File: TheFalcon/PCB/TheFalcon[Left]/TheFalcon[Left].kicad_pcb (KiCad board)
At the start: 4 copper layers, 173.3 x 142.5 mm, 171 parts, among them IC1 IS31FL3729-QFLS4-TR, J2 Conn_01x04_Pin, J3 Conn_01x04_Pin, J5 Conn_01x01, J6 Conn_01x01, SW1 SW_Push, SW2 SW_Push, U2 USBLC6-2P6, U3 USBLC6-2P6, U4 AMS1117-3.3, U6 STM32G431CBTx, Y1 X322516MOB4SI

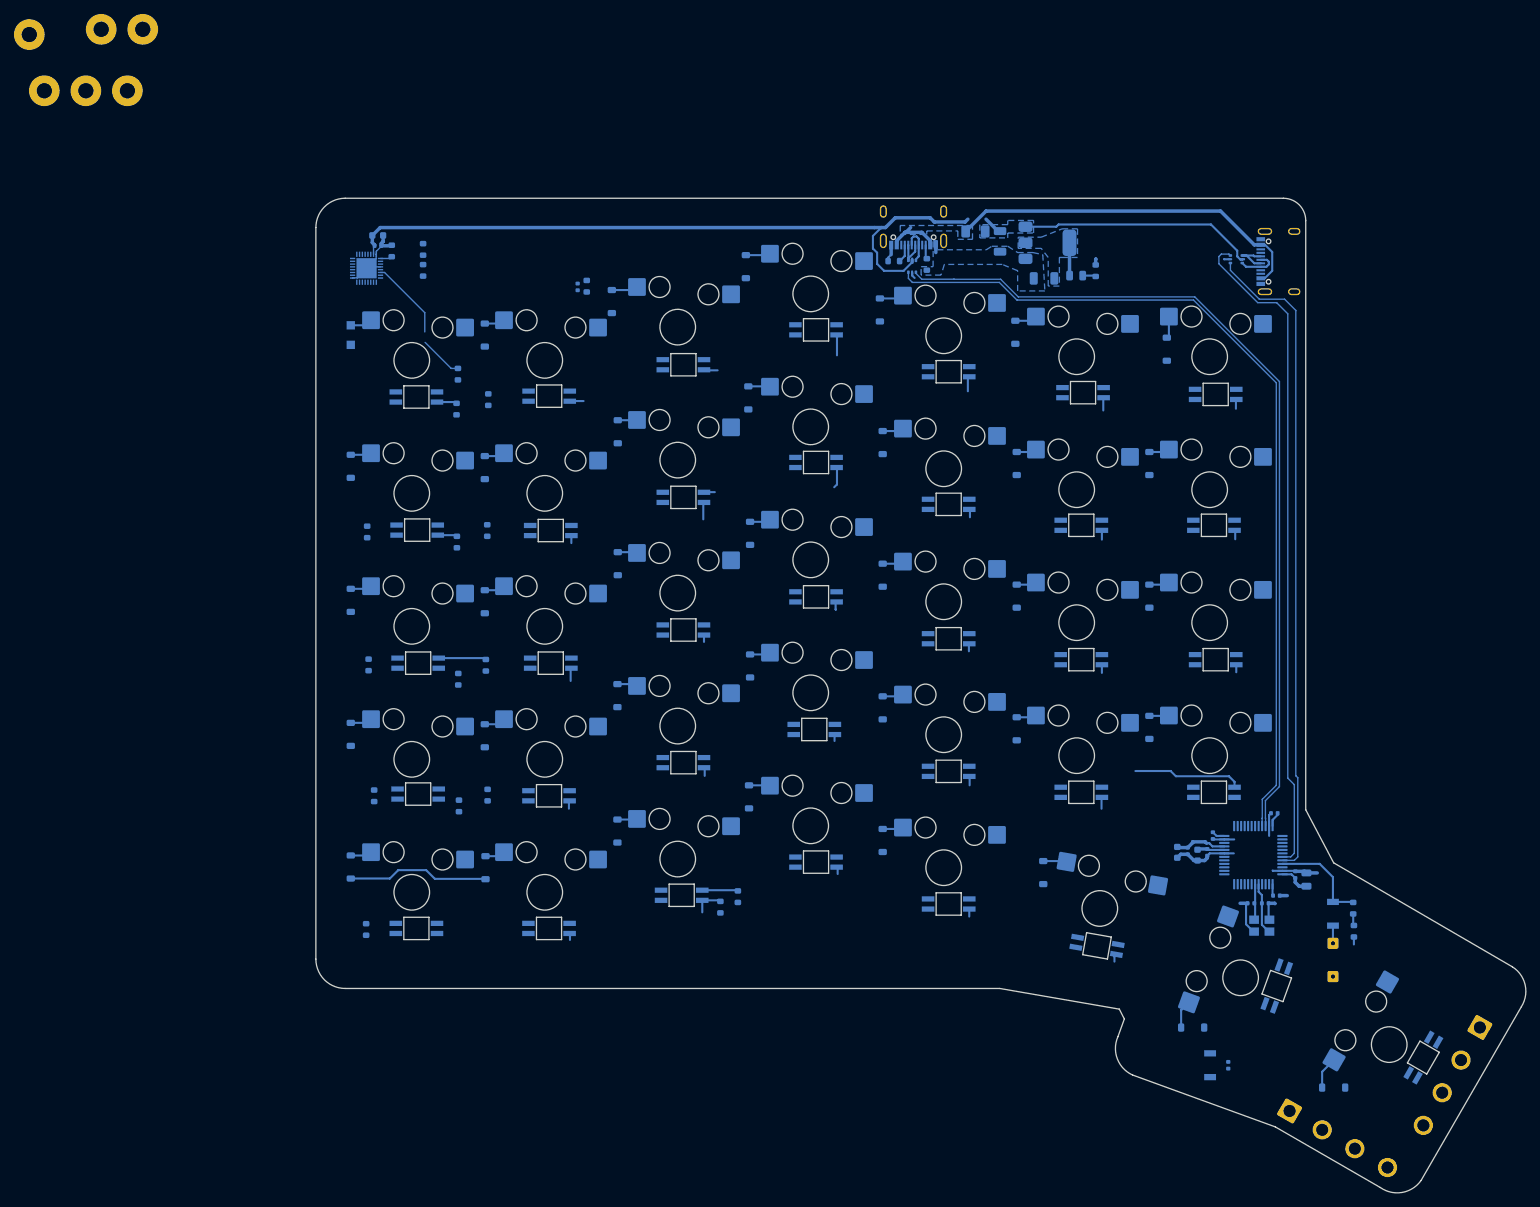
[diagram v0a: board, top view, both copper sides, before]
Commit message: Save
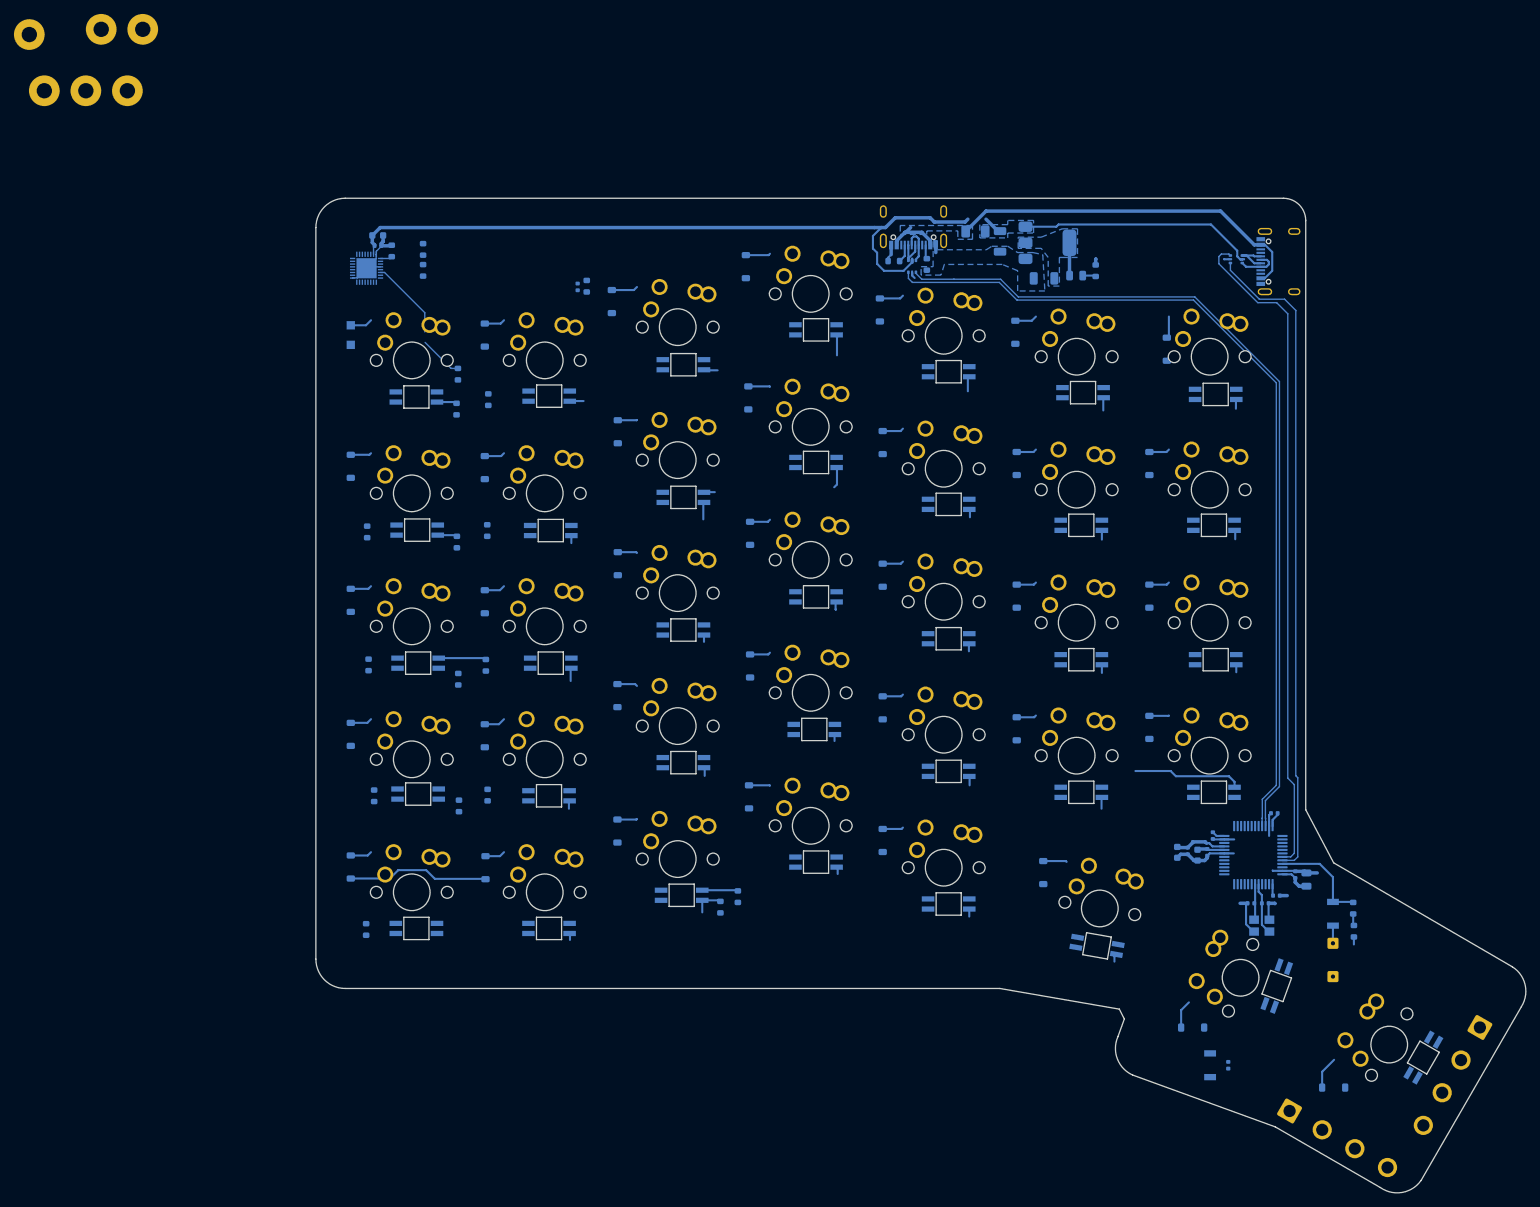
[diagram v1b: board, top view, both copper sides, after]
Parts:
- S1, S10, S11, S12, S13, S14, S15, S16, S17, S18, S19, S2, S20, S21, S22, S23, S24, S25, S26, S27, S28, S29, S3, S30, S31, S32, S33, S34, S4, S5, S6, S7, S8, S9: footprint Gateron_KS33_Hotswap:Gateron-KS33-Hotswap-1U_Model -> MX_KS33:MX_KS33-Solderable-1U; moved to F.Cu
- S35, S36: footprint Gateron_KS33_Hotswap:Gateron-KS33-Hotswap-1.5U -> MX_KS33:MX_KS33-Solderable-1.5U; moved to F.Cu
